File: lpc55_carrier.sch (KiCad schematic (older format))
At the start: 50 parts, among them J101 Conn_2Rows-51Pins, U101 LPC55S28JBD64, Y101 16MHz, Y102 32.768kHz

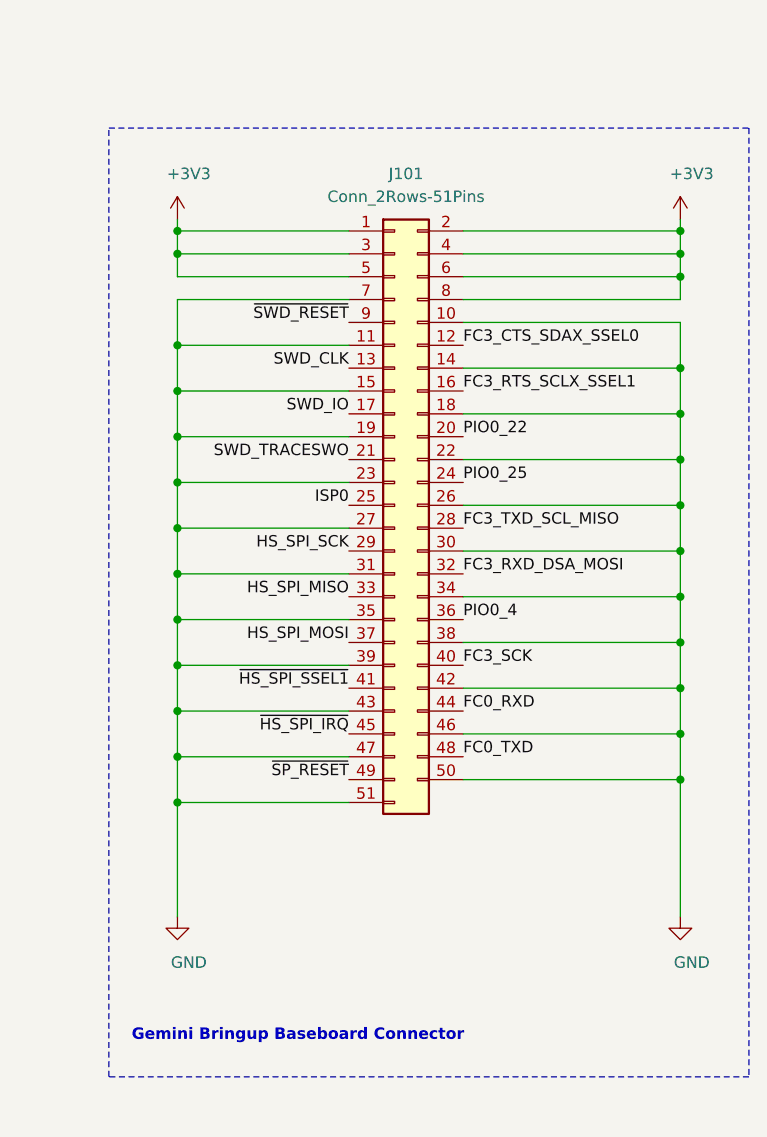
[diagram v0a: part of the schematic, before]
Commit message: lpc55_carrier: rearrange pins on carrier to board connector to ease routing
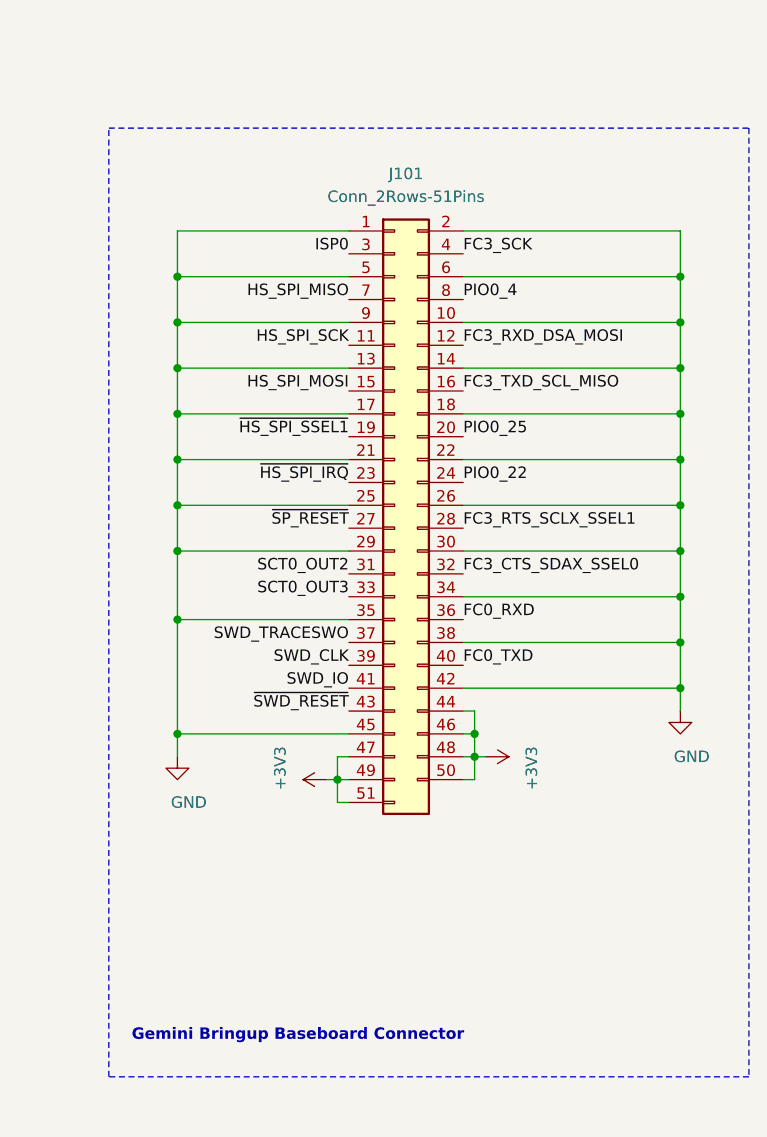
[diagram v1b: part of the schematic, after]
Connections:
- net +3V3: now also J101.44 (Pin_44), J101.46 (Pin_46), J101.47 (Pin_47), J101.48 (Pin_48), J101.49 (Pin_49), J101.50 (Pin_50), J101.51 (Pin_51); no longer J101.1 (Pin_1), J101.2 (Pin_2), J101.3 (Pin_3), J101.4 (Pin_4), J101.5 (Pin_5), J101.6 (Pin_6), J101.8 (Pin_8)
- net FC0_RXD: now also J101.36 (Pin_36); no longer J101.44 (Pin_44)
- net FC0_TXD: now also J101.40 (Pin_40); no longer J101.48 (Pin_48)
- net FC3_CTS_SDAX_SSEL0: now also J101.32 (Pin_32); no longer J101.12 (Pin_12)
- net FC3_RTS_SCLX_SSEL1: now also J101.28 (Pin_28); no longer J101.16 (Pin_16)
- net FC3_RXD_DSA_MOSI: now also J101.12 (Pin_12); no longer J101.32 (Pin_32)
- net FC3_SCK: now also J101.4 (Pin_4); no longer J101.40 (Pin_40)
- net FC3_TXD_SCL_MISO: now also J101.16 (Pin_16); no longer J101.28 (Pin_28)
- net GND: now also J101.1 (Pin_1), J101.13 (Pin_13), J101.17 (Pin_17), J101.2 (Pin_2), J101.21 (Pin_21), J101.25 (Pin_25), J101.29 (Pin_29), J101.45 (Pin_45), J101.5 (Pin_5), J101.6 (Pin_6), J101.9 (Pin_9); no longer J101.11 (Pin_11), J101.15 (Pin_15), J101.19 (Pin_19), J101.23 (Pin_23), J101.27 (Pin_27), J101.31 (Pin_31), J101.39 (Pin_39), J101.43 (Pin_43), J101.46 (Pin_46), J101.47 (Pin_47), J101.50 (Pin_50), J101.51 (Pin_51), J101.7 (Pin_7)
- net HS_SPI_MISO: now also J101.7 (Pin_7); no longer J101.33 (Pin_33)
- net HS_SPI_MOSI: now also J101.15 (Pin_15); no longer J101.37 (Pin_37)
- net HS_SPI_SCK: now also J101.11 (Pin_11); no longer J101.29 (Pin_29)
- net ISP0: now also J101.3 (Pin_3); no longer J101.25 (Pin_25)
- net PIO0_22: now also J101.24 (Pin_24); no longer J101.20 (Pin_20)
- net PIO0_25: now also J101.20 (Pin_20); no longer J101.24 (Pin_24)
- net PIO0_4: now also J101.8 (Pin_8); no longer J101.36 (Pin_36)
- net SCT0_OUT2: now also J101.31 (Pin_31)
- net SCT0_OUT3: now also J101.33 (Pin_33)
- net SWD_CLK: now also J101.39 (Pin_39); no longer J101.13 (Pin_13)
- net SWD_IO: now also J101.41 (Pin_41); no longer J101.17 (Pin_17)
- net SWD_TRACESWO: now also J101.37 (Pin_37); no longer J101.21 (Pin_21)
- net ~HS_SPI_IRQ: now also J101.23 (Pin_23); no longer J101.45 (Pin_45)
- net ~HS_SPI_SSEL1: now also J101.19 (Pin_19); no longer J101.41 (Pin_41)
- net ~SP_RESET: now also J101.27 (Pin_27); no longer J101.49 (Pin_49)
- net ~SWD_RESET: now also J101.43 (Pin_43); no longer J101.9 (Pin_9)
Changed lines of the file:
@@
 Text Label 5200 8350 0    50   ~ 0
 ~RESET
-Text Label 18550 3550 2    50   ~ 0
+Text Label 18550 5250 2    50   ~ 0
 ~SWD_RESET
-Text Label 18550 3750 2    50   ~ 0
+Text Label 18550 5050 2    50   ~ 0
 SWD_CLK
-Text Label 18550 3950 2    50   ~ 0
+Text Label 18550 5150 2    50   ~ 0
 SWD_IO
-Text Label 18550 4150 2    50   ~ 0
+Text Label 18550 4950 2    50   ~ 0
 SWD_TRACESWO
 $Comp
@@
 NoConn ~ 13150 7350
 NoConn ~ 13150 7450
-Text Label 18550 4350 2    50   ~ 0
+Text Label 18550 3250 2    50   ~ 0
 ISP0
 NoConn ~ 13150 3450
@@
 Text Label 10050 6550 2    50   ~ 0
 SCT0_OUT3
-Text Label 18550 4550 2    50   ~ 0
+Text Label 18550 3650 2    50   ~ 0
 HS_SPI_SCK
-Text Label 18550 4750 2    50   ~ 0
+Text Label 18550 3450 2    50   ~ 0
 HS_SPI_MISO
-Text Label 18550 4950 2    50   ~ 0
+Text Label 18550 3850 2    50   ~ 0
 HS_SPI_MOSI
-Text Label 18550 5350 2    50   ~ 0
+Text Label 18550 4250 2    50   ~ 0
 ~HS_SPI_IRQ
-Text Label 18550 5150 2    50   ~ 0
+Text Label 18550 4050 2    50   ~ 0
 ~HS_SPI_SSEL1
-Text Label 18550 5550 2    50   ~ 0
+Text Label 18550 4450 2    50   ~ 0
 ~SP_RESET
-Text Label 19050 3650 0    50   ~ 0
+Text Label 19050 4650 0    50   ~ 0
 FC3_CTS_SDAX_SSEL0
-Text Label 19050 3850 0    50   ~ 0
+Text Label 19050 4450 0    50   ~ 0
 FC3_RTS_SCLX_SSEL1
+Text Label 19050 4050 0    50   ~ 0
+PIO0_25
 Text Label 19050 4250 0    50   ~ 0
-PIO0_25
-Text Label 19050 4050 0    50   ~ 0
 PIO0_22
 Text Label 10050 5650 2    50   ~ 0
 PIO0_22
-Text Label 19050 4450 0    50   ~ 0
+Text Label 19050 3850 0    50   ~ 0
 FC3_TXD_SCL_MISO
-Text Label 19050 4650 0    50   ~ 0
+Text Label 19050 3650 0    50   ~ 0
 FC3_RXD_DSA_MOSI
+Text Label 19050 3450 0    50   ~ 0
+PIO0_4
+Text Label 19050 3250 0    50   ~ 0
+FC3_SCK
 Text Label 19050 4850 0    50   ~ 0
-PIO0_4
+FC0_RXD
 Text Label 19050 5050 0    50   ~ 0
-FC3_SCK
-Text Label 19050 5250 0    50   ~ 0
-FC0_RXD
-Text Label 19050 5450 0    50   ~ 0
 FC0_TXD
 NoConn ~ 10050 3450
@@
 NoConn ~ 10050 6250
 Wire Wire Line
-	18550 3350 17800 3350
-Wire Wire Line
-	17800 3350 17800 3250
-Wire Wire Line
-	18550 3250 17800 3250
-Connection ~ 17800 3250
-Wire Wire Line
-	17800 3250 17800 3150
-Wire Wire Line
-	18550 3150 17800 3150
-Connection ~ 17800 3150
-Wire Wire Line
-	17800 3150 17800 3100
+	18550 5650 18500 5650
+Wire Wire Line
+	18500 5650 18500 5550
+Wire Wire Line
+	18550 5550 18500 5550
+Connection ~ 18500 5550
+Wire Wire Line
+	18500 5550 18500 5450
+Wire Wire Line
+	18550 5450 18500 5450
 $Comp
 L power:+3V3 #PWR0105
 U 1 1 5F4E8259
-P 17800 3100
-F 0 "#PWR0105" H 17800 2950 50  0001 C CNN
-F 1 "+3V3" H 17850 3300 50  0000 C CNN
-F 2 "" H 17800 3100 50  0001 C CNN
-F 3 "" H 17800 3100 50  0001 C CNN
-	1    17800 3100
-	1    0    0    -1
-$EndComp
-Wire Wire Line
-	19050 3450 20000 3450
-Wire Wire Line
-	20000 3450 20000 3350
-Wire Wire Line
-	19050 3350 20000 3350
-Connection ~ 20000 3350
-Wire Wire Line
-	20000 3350 20000 3250
-Wire Wire Line
-	19050 3250 20000 3250
-Connection ~ 20000 3250
-Wire Wire Line
-	20000 3250 20000 3150
-Connection ~ 20000 3150
-Wire Wire Line
-	20000 3150 20000 3100
-Wire Wire Line
-	19050 3150 20000 3150
+P 18450 5550
+F 0 "#PWR0105" H 18450 5400 50  0001 C CNN
+F 1 "+3V3" H 18500 5750 50  0000 C CNN
+F 2 "" H 18450 5550 50  0001 C CNN
+F 3 "" H 18450 5550 50  0001 C CNN
+	1    18450 5550
+	0    -1   -1   0
+$EndComp
+Wire Wire Line
+	19050 5550 19100 5550
+Wire Wire Line
+	19100 5550 19100 5450
+Wire Wire Line
+	19050 5450 19100 5450
+Connection ~ 19100 5450
+Wire Wire Line
+	19100 5450 19100 5350
+Wire Wire Line
+	19050 5350 19100 5350
+Connection ~ 19100 5350
+Wire Wire Line
+	19100 5350 19100 5250
+Wire Wire Line
+	19050 5250 19100 5250
 $Comp
 L power:+3V3 #PWR0106
 U 1 1 5F515ABE
-P 20000 3100
-F 0 "#PWR0106" H 20000 2950 50  0001 C CNN
-F 1 "+3V3" H 20050 3300 50  0000 C CNN
-F 2 "" H 20000 3100 50  0001 C CNN
-F 3 "" H 20000 3100 50  0001 C CNN
-	1    20000 3100
-	1    0    0    -1
-$EndComp
-Wire Wire Line
-	18550 3650 17800 3650
-Wire Wire Line
-	19050 3750 20000 3750
-Wire Wire Line
-	20000 3750 20000 3950
-Wire Wire Line
-	18550 3850 17800 3850
-Connection ~ 17800 3850
-Wire Wire Line
-	17800 3850 17800 4050
-Wire Wire Line
-	18550 4050 17800 4050
-Connection ~ 17800 4050
-Wire Wire Line
-	17800 4050 17800 4250
-Wire Wire Line
-	18550 4250 17800 4250
-Connection ~ 17800 4250
-Wire Wire Line
-	17800 4250 17800 4450
-Wire Wire Line
-	18550 4450 17800 4450
-Connection ~ 17800 4450
-Wire Wire Line
-	17800 4450 17800 4650
-Wire Wire Line
-	18550 4650 17800 4650
-Connection ~ 17800 4650
-Wire Wire Line
-	17800 4650 17800 4850
-Wire Wire Line
-	18550 4850 17800 4850
-Connection ~ 17800 4850
-Wire Wire Line
-	17800 4850 17800 5050
-Wire Wire Line
-	18550 5050 17800 5050
-Connection ~ 17800 5050
-Wire Wire Line
-	17800 5050 17800 5250
-Wire Wire Line
-	18550 5250 17800 5250
-Connection ~ 17800 5250
-Wire Wire Line
-	17800 5250 17800 5450
-Wire Wire Line
-	18550 5450 17800 5450
-Connection ~ 17800 5450
-Wire Wire Line
-	17800 5450 17800 5650
-Wire Wire Line
-	19050 5550 20000 5550
-Connection ~ 20000 5550
-Wire Wire Line
-	20000 5550 20000 6150
-Wire Wire Line
-	19050 5350 20000 5350
-Connection ~ 20000 5350
-Wire Wire Line
-	20000 5350 20000 5550
+P 19150 5450
+F 0 "#PWR0106" H 19150 5300 50  0001 C CNN
+F 1 "+3V3" H 19200 5650 50  0000 C CNN
+F 2 "" H 19150 5450 50  0001 C CNN
+F 3 "" H 19150 5450 50  0001 C CNN
+	1    19150 5450
+	0    1    1    0
+$EndComp
+Wire Wire Line
+	18550 3350 17800 3350
+Wire Wire Line
+	19050 3350 20000 3350
+Wire Wire Line
+	20000 3350 20000 3550
+Wire Wire Line
+	18550 3550 17800 3550
+Connection ~ 17800 3550
+Wire Wire Line
+	17800 3550 17800 3750
+Wire Wire Line
+	18550 3750 17800 3750
+Connection ~ 17800 3750
+Wire Wire Line
+	17800 3750 17800 3950
+Wire Wire Line
+	18550 3950 17800 3950
+Connection ~ 17800 3950
+Wire Wire Line
+	17800 3950 17800 4150
+Wire Wire Line
+	18550 4150 17800 4150
+Connection ~ 17800 4150
+Wire Wire Line
+	17800 4150 17800 4350
+Wire Wire Line
+	18550 4350 17800 4350
+Connection ~ 17800 4350
+Wire Wire Line
+	17800 4350 17800 4550
+Wire Wire Line
+	18550 4550 17800 4550
+Connection ~ 17800 4550
 Wire Wire Line
 	19050 5150 20000 5150
 Connection ~ 20000 5150
 Wire Wire Line
-	20000 5150 20000 5350
+	20000 5150 20000 5250
 Wire Wire Line
 	19050 4950 20000 4950
@@
 Wire Wire Line
 	20000 3950 20000 4150
+Wire Wire Line
+	19050 3750 20000 3750
+Connection ~ 20000 3750
+Wire Wire Line
+	20000 3750 20000 3950
+Wire Wire Line
+	19050 3550 20000 3550
+Connection ~ 20000 3550
+Wire Wire Line
+	20000 3550 20000 3750
 $Comp
 L power:GND #PWR0112
 U 1 1 5F63867A
-P 20000 6150
-F 0 "#PWR0112" H 20000 5900 50  0001 C CNN
-F 1 "GND" H 20050 5950 50  0000 C CNN
-F 2 "" H 20000 6150 50  0001 C CNN
-F 3 "" H 20000 6150 50  0001 C CNN
-	1    20000 6150
+P 20000 5250
+F 0 "#PWR0112" H 20000 5000 50  0001 C CNN
+F 1 "GND" H 20050 5050 50  0000 C CNN
+F 2 "" H 20000 5250 50  0001 C CNN
+F 3 "" H 20000 5250 50  0001 C CNN
+	1    20000 5250
 	1    0    0    -1
 $EndComp
@@
 L power:GND #PWR0111
 U 1 1 5F6388A0
-P 17800 6150
-F 0 "#PWR0111" H 17800 5900 50  0001 C CNN
-F 1 "GND" H 17850 5950 50  0000 C CNN
-F 2 "" H 17800 6150 50  0001 C CNN
-F 3 "" H 17800 6150 50  0001 C CNN
-	1    17800 6150
-	1    0    0    -1
-$EndComp
-Wire Wire Line
-	18550 3450 17800 3450
-Wire Wire Line
-	17800 3450 17800 3650
-Connection ~ 17800 3650
-Wire Wire Line
-	17800 3650 17800 3850
-Wire Wire Line
-	19050 3550 20000 3550
-Wire Wire Line
-	20000 3550 20000 3750
-Connection ~ 20000 3750
+P 17800 5450
+F 0 "#PWR0111" H 17800 5200 50  0001 C CNN
+F 1 "GND" H 17850 5250 50  0000 C CNN
+F 2 "" H 17800 5450 50  0001 C CNN
+F 3 "" H 17800 5450 50  0001 C CNN
+	1    17800 5450
+	1    0    0    -1
+$EndComp
+Wire Wire Line
+	18550 3150 17800 3150
+Wire Wire Line
+	17800 3150 17800 3350
+Connection ~ 17800 3350
+Wire Wire Line
+	17800 3350 17800 3550
+Wire Wire Line
+	19050 3150 20000 3150
+Wire Wire Line
+	20000 3150 20000 3350
+Connection ~ 20000 3350
 Text Notes 17600 6700 0    50   ~ 10
 Gemini Bringup Baseboard Connector
@@
 $EndComp
 Wire Wire Line
-	18550 5650 17800 5650
-Connection ~ 17800 5650
-Wire Wire Line
-	17800 5650 17800 6150
+	18550 5350 17800 5350
+Connection ~ 17800 5350
+Wire Wire Line
+	17800 5350 17800 5450
 Connection ~ 4300 8350
 Wire Wire Line
@@
 	2250 2950 2700 2950
 Connection ~ 2700 2950
+Wire Wire Line
+	19100 5450 19150 5450
+Wire Wire Line
+	18500 5550 18450 5550
+Wire Wire Line
+	17800 4550 17800 4850
+Wire Wire Line
+	18550 4850 17800 4850
+Connection ~ 17800 4850
+Wire Wire Line
+	17800 4850 17800 5350
+Text Label 18550 4750 2    50   ~ 0
+SCT0_OUT3
+Text Label 18550 4650 2    50   ~ 0
+SCT0_OUT2
 $EndSCHEMATC
